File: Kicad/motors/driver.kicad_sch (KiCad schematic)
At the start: 60 parts, among them IC201 L298P, IC202 SN74LVC1G19, IC203 SN74LVC1G19, IC204 L298P, IC205 SN74LVC1G19, IC206 SN74LVC1G19, IC207 LM3480-50, K201 MOTOR 1, K202 MOTOR 2, K203 MOTOR 4, K204 MOTOR 3

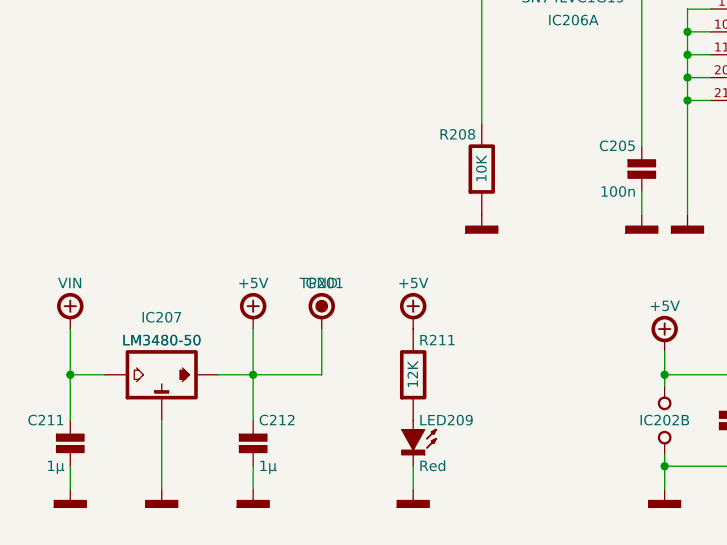
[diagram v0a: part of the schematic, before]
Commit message: Update
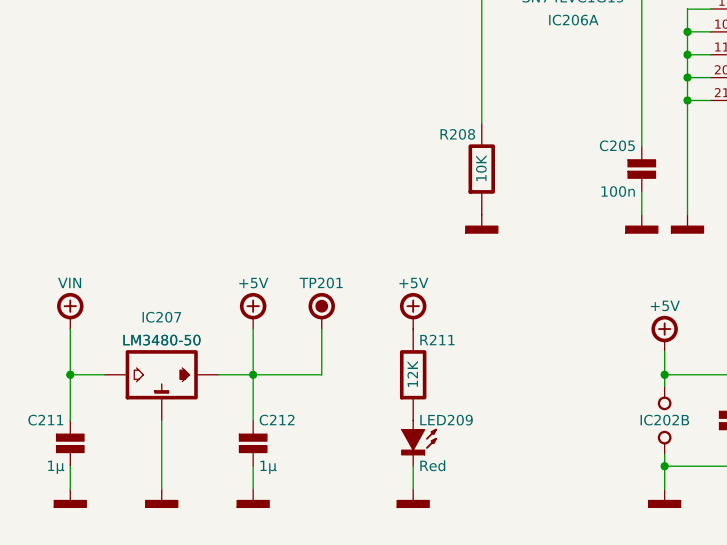
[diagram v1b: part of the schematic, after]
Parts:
- TP201: footprint tronixio:HARWIN-S1751 -> tronixio:zzzHARWIN-S1751; Name GND -> (none)
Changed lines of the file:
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@@
       (effects (font (size 1 1)) hide)
     )
-    (property "Footprint" "tronixio:HARWIN-S1751" (id 2) (at 53.34 177.8 0)
+    (property "Footprint" "tronixio:zzzHARWIN-S1751" (id 2) (at 53.34 177.8 0)
       (effects (font (size 1 1)) hide)
     )
@@
       (effects (font (size 1 1)) hide)
     )
-    (property "Name" "GND" (id 5) (at 53.34 162.56 0)
-      (effects (font (size 1.15 1.15)))
-    )
     (pin "1")
